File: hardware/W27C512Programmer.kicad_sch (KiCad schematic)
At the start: 104 parts, among them J1 CTRL, J2 MSB, J3 LSB, J4 Ext_UART, J5 OLED, J6 VP, J7 SAO, Q1 MMBT3904, Q2 MMBT3906, Q3 MMBT3904, Q4 MMBT3904, Q5 MMBT3904, Q6 MMBT3906, Q7 MMBT3906, Q8 MMBT3906, SW1 RST, SW2 USR, U1 MIC2288, U2 74HC573, U3 74HC573, U4 74HC573, U5 28/32 pin ROM

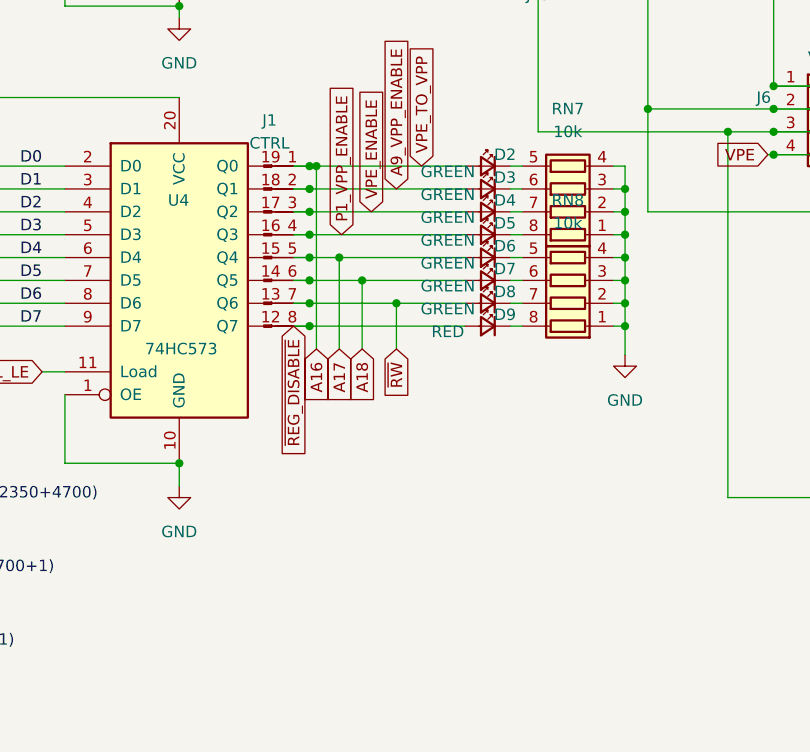
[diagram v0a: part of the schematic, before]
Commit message: Fiddle with pin naming
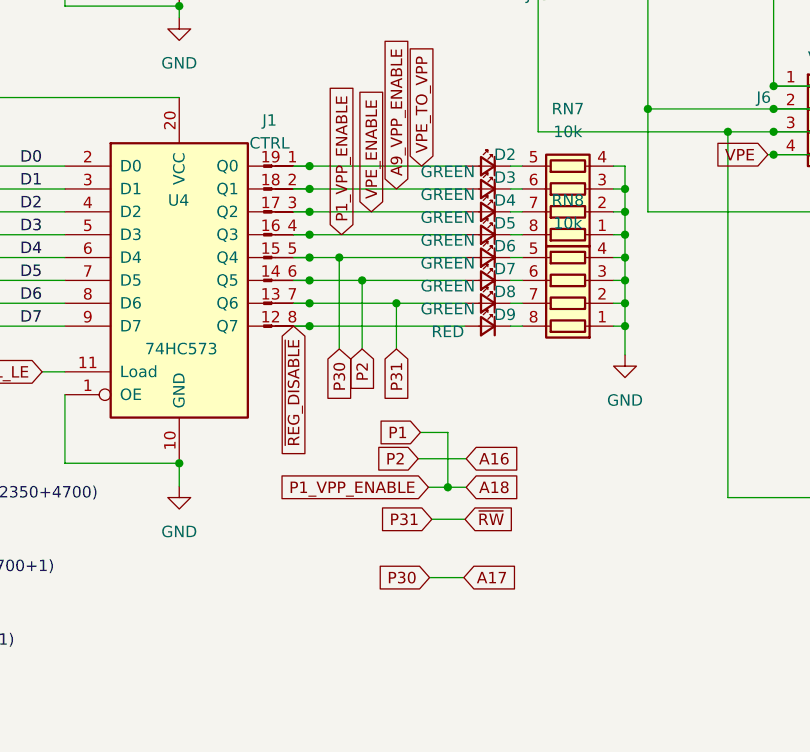
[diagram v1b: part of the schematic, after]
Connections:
- net P1_VPP_ENABLE is gone; now on net A18: D5.2 (A), J1.4 (Pin_4), R25.1, U4.16 (Q3)
- net A16: now also D7.2 (A), J1.6 (Pin_6), U4.14 (Q5); no longer D2.2 (A), J1.1 (Pin_1), R2.1, U4.19 (Q0)
- net A18: no longer D7.2 (A), J1.6 (Pin_6), U4.14 (Q5)
- net ~{RW} renamed P31
- new net VPE_TO_VPP: D2.2 (A), J1.1 (Pin_1), R2.1, U4.19 (Q0)
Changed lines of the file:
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@@
   (junction (at 74.93 62.865) (diameter 0) (color 0 0 0 0)
   )
-  (junction (at 146.05 127) (diameter 0) (color 0 0 0 0)
-  )
   (junction (at 185.42 50.8) (diameter 0) (color 0 0 0 0)
   )
@@
   )
   (junction (at 74.93 32.385) (diameter 0) (color 0 0 0 0)
+  )
+  (junction (at 160.655 162.687) (diameter 0) (color 0 0 0 0)
   )
   (junction (at 194.31 97.79) (diameter 0) (color 0 0 0 0)
@@
     (stroke (width 0) (type default) (color 0 0 0 0))
   )
+  (wire (pts (xy 160.655 156.591) (xy 157.607 156.591))
+    (stroke (width 0) (type default) (color 0 0 0 0))
+  )
   (wire (pts (xy 49.53 96.52) (xy 55.88 96.52))
     (stroke (width 0) (type default) (color 0 0 0 0))
@@
     (stroke (width 0) (type default) (color 0 0 0 0))
   )
-  (wire (pts (xy 146.05 127) (xy 162.56 127))
+  (wire (pts (xy 145.288 127) (xy 162.56 127))
     (stroke (width 0) (type default) (color 0 0 0 0))
   )
@@
     (stroke (width 0) (type default) (color 0 0 0 0))
   )
+  (wire (pts (xy 157.353 159.512) (xy 162.687 159.512))
+    (stroke (width 0) (type default) (color 0 0 0 0))
+  )
   (wire (pts (xy 276.86 144.78) (xy 267.97 144.78))
     (stroke (width 0) (type default) (color 0 0 0 0))
@@
     (stroke (width 0) (type default) (color 0 0 0 0))
   )
+  (wire (pts (xy 158.623 172.72) (xy 162.433 172.72))
+    (stroke (width 0) (type default) (color 0 0 0 0))
+  )
   (wire (pts (xy 34.925 32.385) (xy 52.07 32.385))
     (stroke (width 0) (type default) (color 0 0 0 0))
@@
     (stroke (width 0) (type default) (color 0 0 0 0))
   )
-  (wire (pts (xy 145.288 127) (xy 146.05 127))
-    (stroke (width 0) (type default) (color 0 0 0 0))
-  )
   (wire (pts (xy 55.88 106.68) (xy 62.23 106.68))
     (stroke (width 0) (type default) (color 0 0 0 0))
@@
     (stroke (width 0) (type default) (color 0 0 0 0))
   )
+  (wire (pts (xy 160.655 162.687) (xy 162.687 162.687))
+    (stroke (width 0) (type default) (color 0 0 0 0))
+  )
   (wire (pts (xy 49.53 105.41) (xy 49.53 106.68))
     (stroke (width 0) (type default) (color 0 0 0 0))
@@
     (stroke (width 0) (type default) (color 0 0 0 0))
   )
+  (wire (pts (xy 158.877 166.243) (xy 162.56 166.243))
+    (stroke (width 0) (type default) (color 0 0 0 0))
+  )
   (wire (pts (xy 241.3 91.44) (xy 242.57 91.44))
     (stroke (width 0) (type default) (color 0 0 0 0))
@@
     (stroke (width 0) (type default) (color 0 0 0 0))
   )
+  (wire (pts (xy 160.655 162.687) (xy 160.655 156.591))
+    (stroke (width 0) (type default) (color 0 0 0 0))
+  )
   (wire (pts (xy 74.93 50.165) (xy 74.93 52.705))
     (stroke (width 0) (type default) (color 0 0 0 0))
@@
     (stroke (width 0) (type default) (color 0 0 0 0))
   )
+  (wire (pts (xy 158.496 162.687) (xy 160.655 162.687))
+    (stroke (width 0) (type default) (color 0 0 0 0))
+  )
   (wire (pts (xy 110.49 78.74) (xy 118.11 78.74))
     (stroke (width 0) (type default) (color 0 0 0 0))
@@
   )
   (wire (pts (xy 267.97 125.73) (xy 269.24 125.73))
-    (stroke (width 0) (type default) (color 0 0 0 0))
-  )
-  (wire (pts (xy 146.05 127) (xy 146.05 147.32))
     (stroke (width 0) (type default) (color 0 0 0 0))
   )
@@
     )
   )
-  (global_label "A18" (shape input) (at 151.13 147.32 270) (fields_autoplaced)
-    (effects (font (size 1.27 1.27)) (justify right))
-    (property "Intersheet References" "${INTERSHEET_REFS}" (id 0) (at 151.0506 153.2407 90)
+  (global_label "P2" (shape input) (at 151.13 147.32 270) (fields_autoplaced)
+    (effects (font (size 1.27 1.27)) (justify right))
+    (property "Intersheet References" "${INTERSHEET_REFS}" (id 0) (at 151.0506 152.1237 90)
       (effects (font (size 1.27 1.27)) (justify right) hide)
     )
@@
     )
   )
-  (global_label "A17" (shape input) (at 148.59 147.32 270) (fields_autoplaced)
-    (effects (font (size 1.27 1.27)) (justify right))
-    (property "Intersheet References" "${INTERSHEET_REFS}" (id 0) (at 148.5106 153.2407 90)
+  (global_label "P30" (shape input) (at 148.59 147.32 270) (fields_autoplaced)
+    (effects (font (size 1.27 1.27)) (justify right))
+    (property "Intersheet References" "${INTERSHEET_REFS}" (id 0) (at 148.5106 153.3332 90)
       (effects (font (size 1.27 1.27)) (justify right) hide)
     )
@@
     )
   )
+  (global_label "P2" (shape input) (at 157.353 159.512 180) (fields_autoplaced)
+    (effects (font (size 1.27 1.27)) (justify right))
+    (property "Intersheet References" "${INTERSHEET_REFS}" (id 0) (at 152.5493 159.4326 0)
+      (effects (font (size 1.27 1.27)) (justify right) hide)
+    )
+  )
   (global_label "~{ROM_OE}" (shape input) (at 240.03 53.34 180) (fields_autoplaced)
     (effects (font (size 1.27 1.27)) (justify right))
@@
     (effects (font (size 1.27 1.27)) (justify right))
     (property "Intersheet References" "${INTERSHEET_REFS}" (id 0) (at 178.4833 73.5806 0)
+      (effects (font (size 1.27 1.27)) (justify right) hide)
+    )
+  )
+  (global_label "P1_VPP_ENABLE" (shape input) (at 158.496 162.687 180) (fields_autoplaced)
+    (effects (font (size 1.27 1.27)) (justify right))
+    (property "Intersheet References" "${INTERSHEET_REFS}" (id 0) (at 141.0243 162.7664 0)
       (effects (font (size 1.27 1.27)) (justify right) hide)
     )
@@
     )
   )
+  (global_label "~{RW}" (shape input) (at 162.56 166.243 0) (fields_autoplaced)
+    (effects (font (size 1.27 1.27)) (justify left))
+    (property "Intersheet References" "${INTERSHEET_REFS}" (id 0) (at 167.6945 166.3224 0)
+      (effects (font (size 1.27 1.27)) (justify left) hide)
+    )
+  )
   (global_label "VPE_ENABLE" (shape input) (at 241.3 91.44 180) (fields_autoplaced)
     (effects (font (size 1.27 1.27)) (justify right))
@@
     )
   )
+  (global_label "A17" (shape input) (at 162.433 172.72 0) (fields_autoplaced)
+    (effects (font (size 1.27 1.27)) (justify left))
+    (property "Intersheet References" "${INTERSHEET_REFS}" (id 0) (at 168.3537 172.7994 0)
+      (effects (font (size 1.27 1.27)) (justify left) hide)
+    )
+  )
   (global_label "CTRL_LE" (shape input) (at 240.03 55.88 180) (fields_autoplaced)
     (effects (font (size 1.27 1.27)) (justify right))
     (property "Intersheet References" "${INTERSHEET_REFS}" (id 0) (at 229.9364 55.8006 0)
+      (effects (font (size 1.27 1.27)) (justify right) hide)
+    )
+  )
+  (global_label "P31" (shape input) (at 158.877 166.243 180) (fields_autoplaced)
+    (effects (font (size 1.27 1.27)) (justify right))
+    (property "Intersheet References" "${INTERSHEET_REFS}" (id 0) (at 152.8638 166.1636 0)
       (effects (font (size 1.27 1.27)) (justify right) hide)
     )
@@
     )
   )
-  (global_label "~{RW}" (shape input) (at 154.94 147.32 270) (fields_autoplaced)
-    (effects (font (size 1.27 1.27)) (justify right))
-    (property "Intersheet References" "${INTERSHEET_REFS}" (id 0) (at 154.8606 152.4545 90)
+  (global_label "P31" (shape input) (at 154.94 147.32 270) (fields_autoplaced)
+    (effects (font (size 1.27 1.27)) (justify right))
+    (property "Intersheet References" "${INTERSHEET_REFS}" (id 0) (at 154.8606 153.3332 90)
       (effects (font (size 1.27 1.27)) (justify right) hide)
     )
@@
     (property "Intersheet References" "${INTERSHEET_REFS}" (id 0) (at 308.61 104.14 0)
       (effects (font (size 1.27 1.27)) hide)
+    )
+  )
+  (global_label "P30" (shape input) (at 158.623 172.72 180) (fields_autoplaced)
+    (effects (font (size 1.27 1.27)) (justify right))
+    (property "Intersheet References" "${INTERSHEET_REFS}" (id 0) (at 152.6098 172.6406 0)
+      (effects (font (size 1.27 1.27)) (justify right) hide)
     )
   )
@@
     )
   )
+  (global_label "A18" (shape input) (at 162.687 162.687 0) (fields_autoplaced)
+    (effects (font (size 1.27 1.27)) (justify left))
+    (property "Intersheet References" "${INTERSHEET_REFS}" (id 0) (at 168.6077 162.7664 0)
+      (effects (font (size 1.27 1.27)) (justify left) hide)
+    )
+  )
+  (global_label "P1" (shape input) (at 157.607 156.591 180) (fields_autoplaced)
+    (effects (font (size 1.27 1.27)) (justify right))
+    (property "Intersheet References" "${INTERSHEET_REFS}" (id 0) (at 152.8033 156.5116 0)
+      (effects (font (size 1.27 1.27)) (justify right) hide)
+    )
+  )
   (global_label "RMSBLE" (shape input) (at 118.11 99.06 180) (fields_autoplaced)
     (effects (font (size 1.27 1.27)) (justify right))
@@
     )
   )
-  (global_label "A16" (shape input) (at 146.05 147.32 270) (fields_autoplaced)
-    (effects (font (size 1.27 1.27)) (justify right))
-    (property "Intersheet References" "${INTERSHEET_REFS}" (id 0) (at 145.9706 153.2407 90)
-      (effects (font (size 1.27 1.27)) (justify right) hide)
-    )
-  )
+  (global_label "A16" (shape input) (at 162.687 159.512 0) (fields_autoplaced)
+    (effects (font (size 1.27 1.27)) (justify left))
+    (property "Intersheet References" "${INTERSHEET_REFS}" (id 0) (at 168.6077 159.5914 0)
+      (effects (font (size 1.27 1.27)) (justify left) hide)
+    )
+  )
